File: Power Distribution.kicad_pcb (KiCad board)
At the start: 2 copper layers, 32.5 x 59.4 mm, 16 parts, among them J1 Conn_01x02, J2 Conn_01x02, J3 Conn_01x02, J4 Conn_01x02, Q1 Q_PMOS_DGS

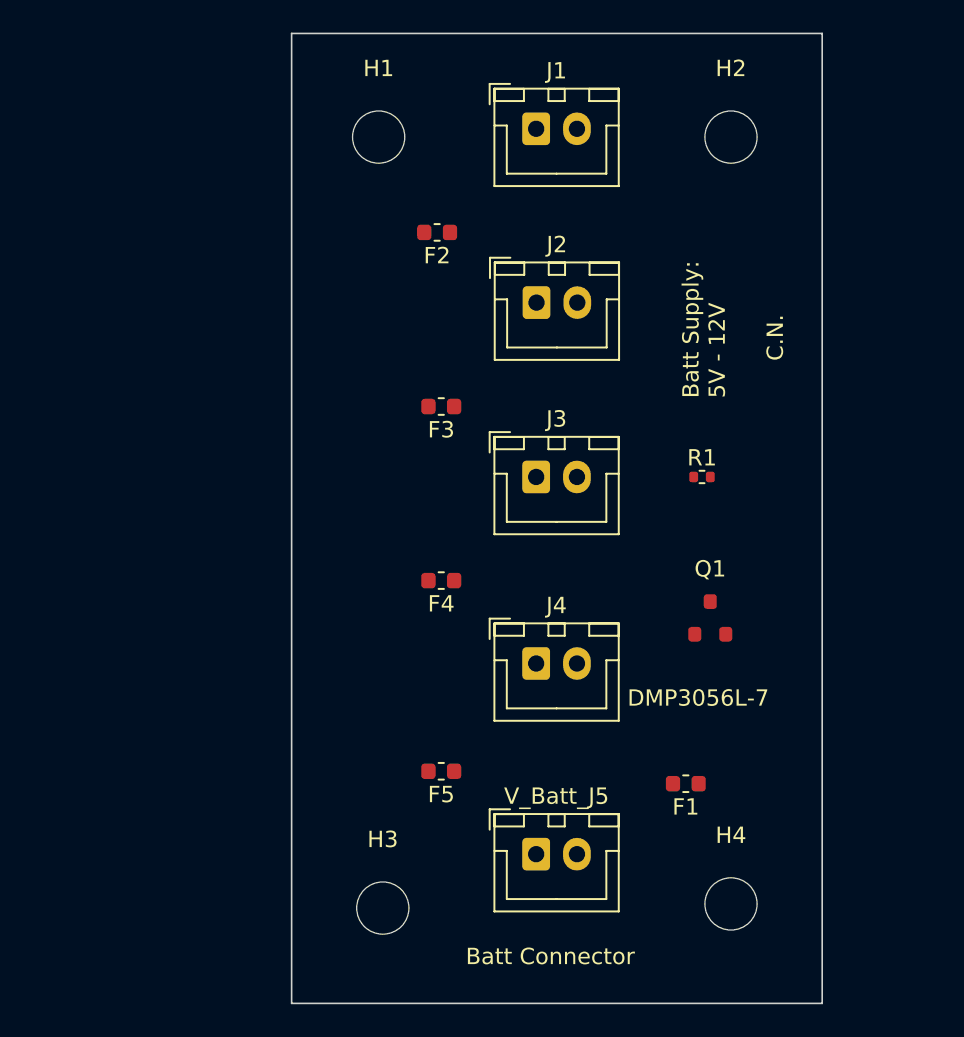
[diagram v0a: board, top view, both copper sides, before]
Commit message: Add files via upload
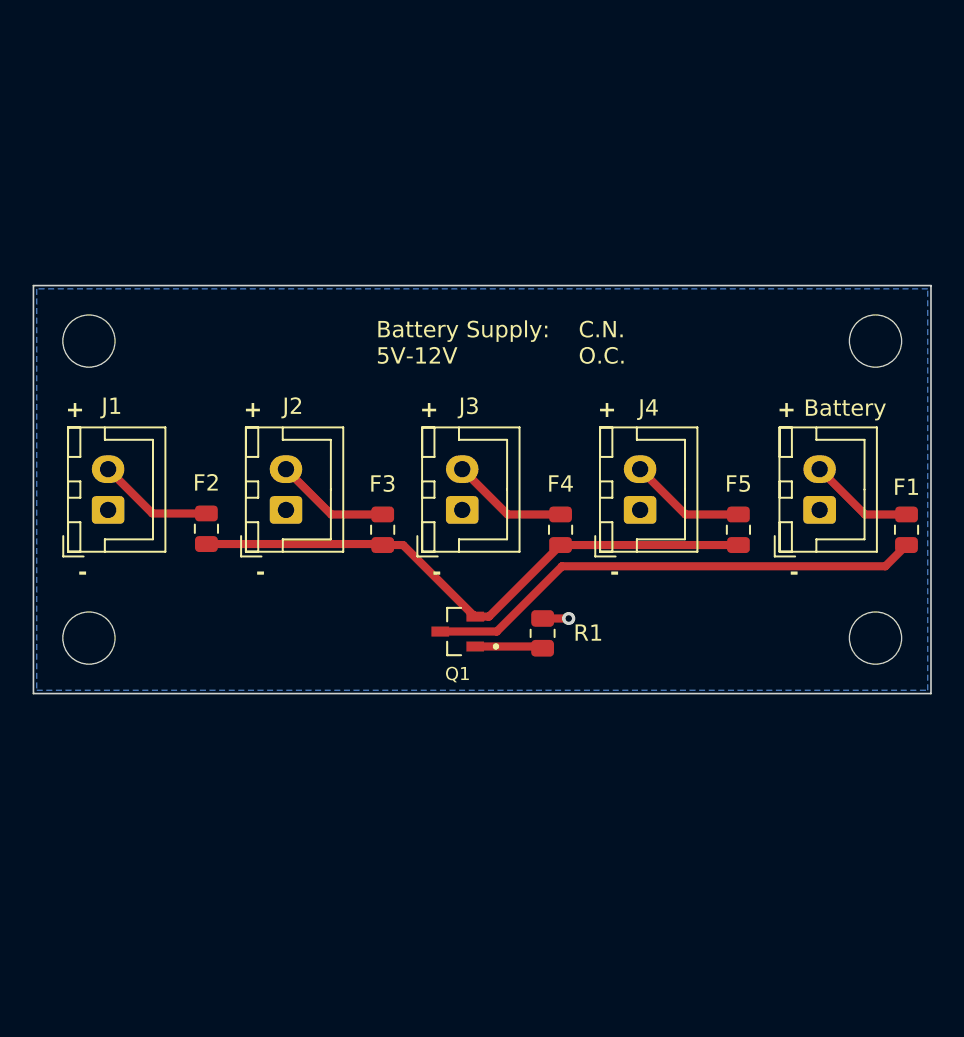
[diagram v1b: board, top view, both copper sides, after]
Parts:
- F1, F2, F4, F5: footprint Fuse:Fuse_0603_1608Metric -> Fuse:Fuse_0805_2012Metric
- F3: value 500 mAFuse -> 500mA Fuse; footprint Fuse:Fuse_0603_1608Metric -> Fuse:Fuse_0805_2012Metric
- Q1: footprint Transistor_Packages:SOT23_Standard -> DMP3056L-7 2:SOT91P240X110-3N
- R1: footprint Resistor_SMD:R_0402_1005Metric -> Resistor_SMD:R_0805_2012Metric
- V_Batt_J5: value Conn_01x02 -> Conn_01x02
- moved H2 41.3 mm to (71.4, 76.0), turned to 90 degrees
- moved H4 35.6 mm to (119.6, 76.0), turned to 90 degrees
- moved H1 35.5 mm to (71.4, 94.2), turned to 90 degrees
- moved J1 35.1 mm to (72.6, 86.3), turned to 90 degrees
- moved H3 34.4 mm to (119.6, 94.2), turned to 90 degrees
- moved V_Batt_J5 27.3 mm to (116.2, 86.3), turned to 90 degrees
- moved F5 23.5 mm to (111.2, 87.6), turned to 90 degrees
- moved F2 23.0 mm to (78.6, 87.5), turned to 90 degrees
- moved F1 20.6 mm to (121.5, 87.6), turned to 90 degrees
- moved J2 19.9 mm to (83.5, 86.3), turned to 90 degrees
- moved Q1 15.5 mm to (94.0, 93.8), turned to 180 degrees
- moved R1 13.7 mm to (99.2, 93.9), turned to 90 degrees
- moved J4 11.4 mm to (105.2, 86.3), turned to 90 degrees
- moved F3 8.36 mm to (89.4, 87.6), turned to 90 degrees
- moved F4 7.95 mm to (100.3, 87.6), turned to 90 degrees
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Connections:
- F1 pad 1: + V_Batt -> Net-(Q1-D)
- F1 pad 2: Net-(Q1-D) -> +VBATT
- F2 pad 1: Net-(J1-Pin_1) -> Net-(Q1-S)
- F2 pad 2: Net-(Q1-S) -> Net-(J1-Pin_2)
- F3 pad 1: Net-(J2-Pin_1) -> Net-(Q1-S)
- F3 pad 2: Net-(Q1-S) -> Net-(J2-Pin_2)
- F4 pad 1: Net-(J3-Pin_1) -> Net-(Q1-S)
- F4 pad 2: Net-(Q1-S) -> Net-(J3-Pin_2)
- F5 pad 1: Net-(J4-Pin_1) -> Net-(Q1-S)
- F5 pad 2: Net-(Q1-S) -> Net-(J4-Pin_2)
- J1 pad 1: Net-(J1-Pin_1) -> GND
- J1 pad 2: - V_BATT -> Net-(J1-Pin_2)
- J2 pad 1: Net-(J2-Pin_1) -> GND
- J2 pad 2: - V_BATT -> Net-(J2-Pin_2)
- J3 pad 1: Net-(J3-Pin_1) -> GND
- J3 pad 2: - V_BATT -> Net-(J3-Pin_2)
- J4 pad 1: Net-(J4-Pin_1) -> GND
- J4 pad 2: - V_BATT -> Net-(J4-Pin_2)
- R1 pad 2: - V_BATT -> GND
- V_Batt_J5 pad 1: + V_Batt -> GND
- V_Batt_J5 pad 2: - V_BATT -> +VBATT
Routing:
- net Net-(Q1-S): track 0.00 -> 36.3 mm
- net Net-(Q1-D): track 0.00 -> 30.8 mm
- net Net-(J4-Pin_2): track 0.00 -> 7.17 mm
- net Net-(J3-Pin_2): track 0.00 -> 7.17 mm
- net Net-(J1-Pin_2): track 0.00 -> 7.15 mm
- net Net-(J2-Pin_2): track 0.00 -> 7.07 mm
- net +VBATT: track 0.00 -> 6.47 mm
- net Net-(Q1-G): track 0.00 -> 3.88 mm
- net GND: track 0.00 -> 1.60 mm, vias 0 -> 1
- added copper zone on B.Cu, net GND
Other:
- board size 32.5 x 59.4 mm -> 55 x 25 mm
- board text added: "+"
- board text added: "-"
- board text added: "Battery"
- board text added: "Battery Supply: 5V-12V"
- board text added: "C.N. O.C."
- board text removed: "Batt Connector"
- board text removed: "Batt Supply: 5V - 12V"
- board text removed: "C.N."
